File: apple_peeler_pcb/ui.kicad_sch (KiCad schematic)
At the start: 6 parts, among them SW3 SPST BTN

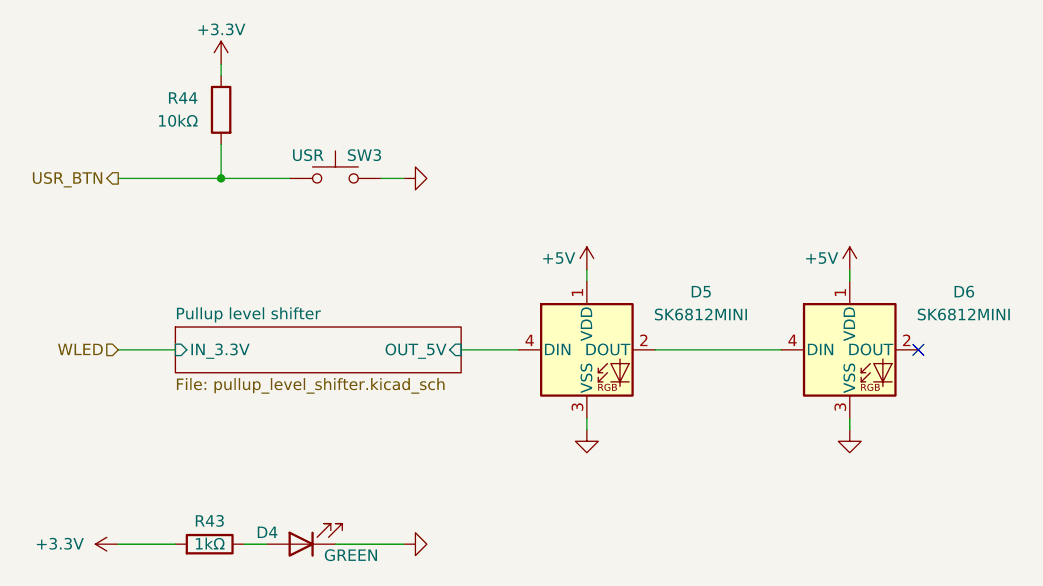
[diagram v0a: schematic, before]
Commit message: fix the fucking WLED footprints
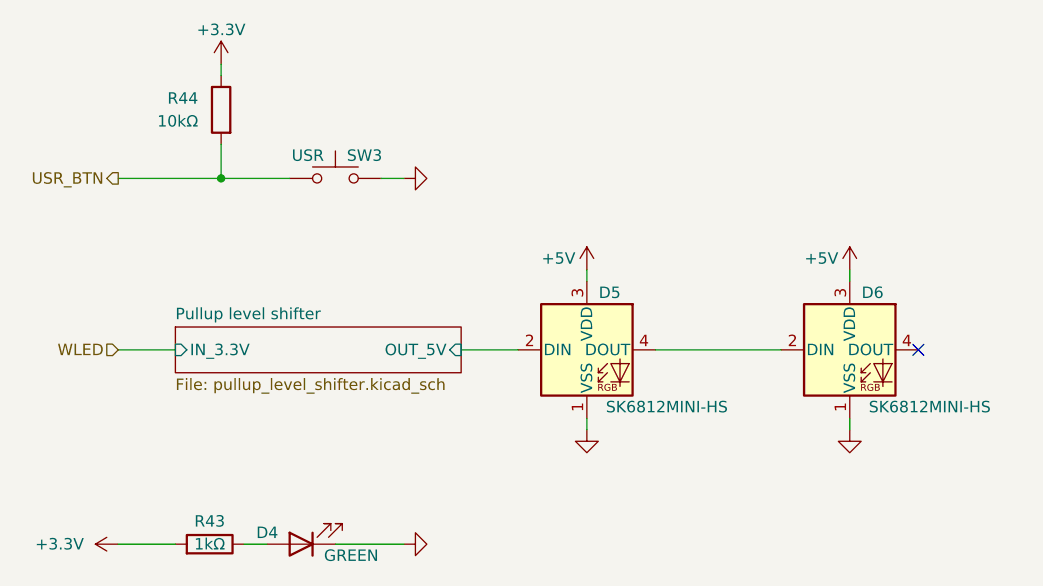
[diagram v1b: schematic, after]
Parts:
- removed D5, D6: SK6812MINI, LED_SMD:LED_SK6812MINI_PLCC4_3.5x3.5mm_P1.75mm, symbol led:SK6812MINI
- added D5, D6: SK6812MINI-HS, leds:LED_SK6812MINI_HS_012, symbol LED:SK6812
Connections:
- net +5V: now also D5.3 (VDD), D6.3 (VDD)
- net GND: now also D5.1 (VSS), D6.1 (VSS)
- net Pullup level shifter/OUT_5V: now also D5.2 (DIN)
- new net: D5.4 (DOUT), D6.2 (DIN)
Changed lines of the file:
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@@
+	)
+	(symbol
+		(lib_id "LED:SK6812")
+		(at 184.15 110.49 0)
+		(unit 1)
+		(exclude_from_sim no)
+		(in_bom yes)
+		(on_board yes)
+		(dnp no)
+		(property "Reference" "D5"
+			(at 186.69 104.14 0)
+			(effects
+				(font
+					(size 1.27 1.27)
+				)
+			)
+		)
+		(property "Value" "SK6812MINI-HS"
+			(at 193.04 116.84 0)
+			(effects
+				(font
+					(size 1.27 1.27)
+				)
+			)
+		)
+		(property "Footprint" "leds:LED_SK6812MINI_HS_012"
+			(at 185.42 118.11 0)
+			(effects
+				(font
+					(size 1.27 1.27)
+				)
+				(justify left top)
+				(hide yes)
+			)
+		)
+		(property "Datasheet" "https://cdn-shop.adafruit.com/product-files/1138/SK6812+LED+datasheet+.pdf"
+			(at 186.69 120.015 0)
+			(effects
+				(font
+					(size 1.27 1.27)
+				)
+				(justify left top)
+				(hide yes)
+			)
+		)
+		(property "Description" "RGB LED with integrated controller"
+			(at 184.15 110.49 0)
+			(effects
+				(font
+					(size 1.27 1.27)
+				)
+				(hide yes)
+			)
+		)
+		(property "MPN" "SK6812MINI-HS"
+			(at 184.15 110.49 0)
+			(effects
+				(font
+					(size 1.27 1.27)
+				)
+				(hide yes)
+			)
+		)
+		(property "LCSC" "C2922787"
+			(at 184.15 110.49 0)
+			(effects
+				(font
+					(size 1.27 1.27)
+				)
+				(hide yes)
+			)
+		)
+		(pin "4"
+		)
+		(pin "1"
+		)
+		(pin "3"
+		)
+		(pin "2"
+		)
+		(instances
+			(project ""
+				(path "/d5946b96-44a8-4a28-8641-19803e1510af/ff7927ce-242d-46a3-8944-ca0e798b7163"
+					(reference "D5")
+					(unit 1)
+				)
+			)
+		)
 	)
 	(symbol
@@
 				(path "/d5946b96-44a8-4a28-8641-19803e1510af/ff7927ce-242d-46a3-8944-ca0e798b7163"
 					(reference "#PWR0101")
-					(unit 1)
-				)
-			)
-		)
-	)
-	(symbol
-		(lib_id "led:SK6812MINI")
-		(at 213.36 110.49 0)
-		(unit 1)
-		(exclude_from_sim no)
-		(in_bom yes)
-		(on_board yes)
-		(dnp no)
-		(fields_autoplaced yes)
-		(property "Reference" "D6"
-			(at 226.06 104.0698 0)
-			(effects
-				(font
-					(size 1.27 1.27)
-				)
-			)
-		)
-		(property "Value" "SK6812MINI"
-			(at 226.06 106.6098 0)
-			(effects
-				(font
-					(size 1.27 1.27)
-				)
-			)
-		)
-		(property "Footprint" "LED_SMD:LED_SK6812MINI_PLCC4_3.5x3.5mm_P1.75mm"
-			(at 214.63 118.11 0)
-			(effects
-				(font
-					(size 1.27 1.27)
-				)
-				(justify left top)
-				(hide yes)
-			)
-		)
-		(property "Datasheet" "https://cdn-shop.adafruit.com/product-files/2686/SK6812MINI_REV.01-1-2.pdf"
-			(at 215.9 120.015 0)
-			(effects
-				(font
-					(size 1.27 1.27)
-				)
-				(justify left top)
-				(hide yes)
-			)
-		)
-		(property "Description" "RGB LED with integrated controller"
-			(at 213.36 110.49 0)
-			(effects
-				(font
-					(size 1.27 1.27)
-				)
-				(hide yes)
-			)
-		)
-		(property "Part" ""
-			(at 213.36 110.49 0)
-			(effects
-				(font
-					(size 1.27 1.27)
-				)
-				(hide yes)
-			)
-		)
-		(property "LCSC" "C5149201"
-			(at 213.36 110.49 0)
-			(effects
-				(font
-					(size 1.27 1.27)
-				)
-				(hide yes)
-			)
-		)
-		(property "MPN" "SK6812MINI-E"
-			(at 213.36 110.49 0)
-			(effects
-				(font
-					(size 1.27 1.27)
-				)
-				(hide yes)
-			)
-		)
-		(pin "2"
-		)
-		(pin "4"
-		)
-		(pin "3"
-		)
-		(pin "1"
-		)
-		(instances
-			(project "apple_peeler_pcb"
-				(path "/d5946b96-44a8-4a28-8641-19803e1510af/ff7927ce-242d-46a3-8944-ca0e798b7163"
-					(reference "D6")
 					(unit 1)
 				)
@@
 	)
 	(symbol
-		(lib_id "led:SK6812MINI")
-		(at 184.15 110.49 0)
-		(unit 1)
-		(exclude_from_sim no)
-		(in_bom yes)
-		(on_board yes)
-		(dnp no)
-		(fields_autoplaced yes)
-		(property "Reference" "D5"
-			(at 196.85 104.0698 0)
-			(effects
-				(font
-					(size 1.27 1.27)
-				)
-			)
-		)
-		(property "Value" "SK6812MINI"
-			(at 196.85 106.6098 0)
-			(effects
-				(font
-					(size 1.27 1.27)
-				)
-			)
-		)
-		(property "Footprint" "LED_SMD:LED_SK6812MINI_PLCC4_3.5x3.5mm_P1.75mm"
-			(at 185.42 118.11 0)
-			(effects
-				(font
-					(size 1.27 1.27)
-				)
-				(justify left top)
-				(hide yes)
-			)
-		)
-		(property "Datasheet" "https://cdn-shop.adafruit.com/product-files/2686/SK6812MINI_REV.01-1-2.pdf"
-			(at 186.69 120.015 0)
-			(effects
-				(font
-					(size 1.27 1.27)
-				)
-				(justify left top)
-				(hide yes)
-			)
-		)
-		(property "Description" "RGB LED with integrated controller"
-			(at 184.15 110.49 0)
-			(effects
-				(font
-					(size 1.27 1.27)
-				)
-				(hide yes)
-			)
-		)
-		(property "Part" ""
-			(at 184.15 110.49 0)
-			(effects
-				(font
-					(size 1.27 1.27)
-				)
-				(hide yes)
-			)
-		)
-		(property "LCSC" "C5149201"
-			(at 184.15 110.49 0)
-			(effects
-				(font
-					(size 1.27 1.27)
-				)
-				(hide yes)
-			)
-		)
-		(property "MPN" "SK6812MINI-E"
-			(at 184.15 110.49 0)
-			(effects
-				(font
-					(size 1.27 1.27)
-				)
-				(hide yes)
-			)
-		)
-		(pin "2"
-		)
-		(pin "4"
-		)
-		(pin "3"
-		)
-		(pin "1"
-		)
-		(instances
-			(project "apple_peeler_pcb"
-				(path "/d5946b96-44a8-4a28-8641-19803e1510af/ff7927ce-242d-46a3-8944-ca0e798b7163"
-					(reference "D5")
-					(unit 1)
-				)
-			)
-		)
-	)
-	(symbol
 		(lib_id "power:GND")
 		(at 213.36 119.38 0)
@@
 					(unit 1)
 				)
+			)
+		)
+	)
+	(symbol
+		(lib_id "LED:SK6812")
+		(at 213.36 110.49 0)
+		(unit 1)
+		(exclude_from_sim no)
+		(in_bom yes)
+		(on_board yes)
+		(dnp no)
+		(property "Reference" "D6"
+			(at 215.9 104.14 0)
+			(effects
+				(font
+					(size 1.27 1.27)
+				)
+			)
+		)
+		(property "Value" "SK6812MINI-HS"
+			(at 222.25 116.84 0)
+			(effects
+				(font
+					(size 1.27 1.27)
+				)
+			)
+		)
+		(property "Footprint" "leds:LED_SK6812MINI_HS_012"
+			(at 214.63 118.11 0)
+			(effects
+				(font
+					(size 1.27 1.27)
+				)
+				(justify left top)
+				(hide yes)
+			)
+		)
+		(property "Datasheet" "https://cdn-shop.adafruit.com/product-files/1138/SK6812+LED+datasheet+.pdf"
+			(at 215.9 120.015 0)
+			(effects
+				(font
+					(size 1.27 1.27)
+				)
+				(justify left top)
+				(hide yes)
+			)
+		)
+		(property "Description" "RGB LED with integrated controller"
+			(at 213.36 110.49 0)
+			(effects
+				(font
+					(size 1.27 1.27)
+				)
+				(hide yes)
+			)
+		)
+		(property "MPN" "SK6812MINI-HS"
+			(at 213.36 110.49 0)
+			(effects
+				(font
+					(size 1.27 1.27)
+				)
+				(hide yes)
+			)
+		)
+		(property "LCSC" "C2922787"
+			(at 213.36 110.49 0)
+			(effects
+				(font
+					(size 1.27 1.27)
+				)
+				(hide yes)
+			)
+		)
+		(pin "4"
+		)
+		(pin "1"
+		)
+		(pin "3"
+		)
+		(pin "2"
+		)
+		(instances
+			(project "apple_peeler_pcb"
+				(path "/d5946b96-44a8-4a28-8641-19803e1510af/ff7927ce-242d-46a3-8944-ca0e798b7163"
+					(reference "D6")
+					(unit 1)
+				)
